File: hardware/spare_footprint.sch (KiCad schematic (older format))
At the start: 37 parts, among them J45 header?, J46 header?, J47 header?, J48 header?, J49 header?

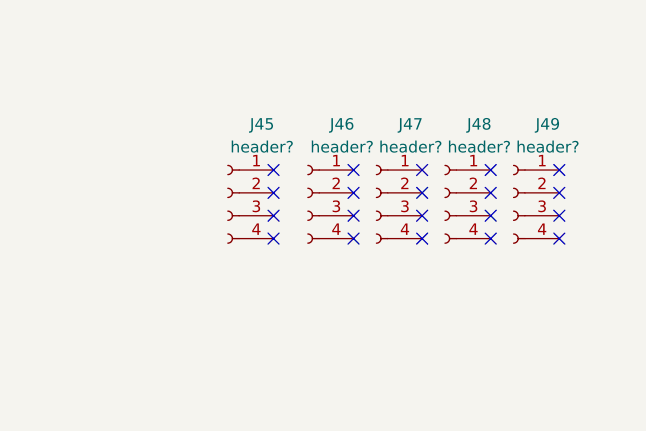
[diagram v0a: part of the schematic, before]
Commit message: update footprint,
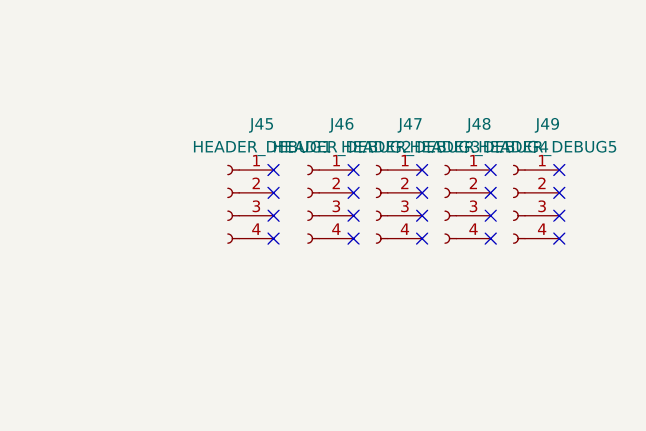
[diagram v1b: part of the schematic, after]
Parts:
- J45: value header? -> HEADER_DEBUG1; footprint (none) -> Connector_PinHeader_1.27mm:PinHeader_1x04_P1.27mm_Vertical
- J46: value header? -> HEADER_DEBUG2; footprint (none) -> Connector_PinHeader_1.27mm:PinHeader_1x04_P1.27mm_Vertical
- J47: value header? -> HEADER_DEBUG3; footprint (none) -> Connector_PinHeader_1.27mm:PinHeader_1x04_P1.27mm_Vertical
- J48: value header? -> HEADER_DEBUG4; footprint (none) -> Connector_PinHeader_1.27mm:PinHeader_1x04_P1.27mm_Vertical
- J49: value header? -> HEADER_DEBUG5; footprint (none) -> Connector_PinHeader_1.27mm:PinHeader_1x04_P1.27mm_Vertical
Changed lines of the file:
@@
 P 3550 1550
 F 0 "J45" H 3400 1850 50  0000 C CNN
-F 1 "header?" H 3400 1750 50  0000 C CNN
-F 2 "" H 3550 1550 50  0001 C CNN
+F 1 "HEADER_DEBUG1" H 3400 1750 50  0000 C CNN
+F 2 "Connector_PinHeader_1.27mm:PinHeader_1x04_P1.27mm_Vertical" H 3550 1550 50  0001 C CNN
 F 3 "~" H 3550 1550 50  0001 C CNN
 	1    3550 1550
@@
 P 3900 1550
 F 0 "J46" H 3750 1850 50  0000 C CNN
-F 1 "header?" H 3750 1750 50  0000 C CNN
-F 2 "" H 3900 1550 50  0001 C CNN
+F 1 "HEADER_DEBUG2" H 3750 1750 50  0000 C CNN
+F 2 "Connector_PinHeader_1.27mm:PinHeader_1x04_P1.27mm_Vertical" H 3900 1550 50  0001 C CNN
 F 3 "~" H 3900 1550 50  0001 C CNN
 	1    3900 1550
@@
 P 4200 1550
 F 0 "J47" H 4050 1850 50  0000 C CNN
-F 1 "header?" H 4050 1750 50  0000 C CNN
-F 2 "" H 4200 1550 50  0001 C CNN
+F 1 "HEADER_DEBUG3" H 4050 1750 50  0000 C CNN
+F 2 "Connector_PinHeader_1.27mm:PinHeader_1x04_P1.27mm_Vertical" H 4200 1550 50  0001 C CNN
 F 3 "~" H 4200 1550 50  0001 C CNN
 	1    4200 1550
@@
 P 4500 1550
 F 0 "J48" H 4350 1850 50  0000 C CNN
-F 1 "header?" H 4350 1750 50  0000 C CNN
-F 2 "" H 4500 1550 50  0001 C CNN
+F 1 "HEADER_DEBUG4" H 4350 1750 50  0000 C CNN
+F 2 "Connector_PinHeader_1.27mm:PinHeader_1x04_P1.27mm_Vertical" H 4500 1550 50  0001 C CNN
 F 3 "~" H 4500 1550 50  0001 C CNN
 	1    4500 1550
@@
 P 4800 1550
 F 0 "J49" H 4650 1850 50  0000 C CNN
-F 1 "header?" H 4650 1750 50  0000 C CNN
-F 2 "" H 4800 1550 50  0001 C CNN
+F 1 "HEADER_DEBUG5" H 4650 1750 50  0000 C CNN
+F 2 "Connector_PinHeader_1.27mm:PinHeader_1x04_P1.27mm_Vertical" H 4800 1550 50  0001 C CNN
 F 3 "~" H 4800 1550 50  0001 C CNN
 	1    4800 1550
